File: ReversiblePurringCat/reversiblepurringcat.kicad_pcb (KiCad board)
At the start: 2 copper layers, 230.3 x 90.7 mm, 78 parts, among them J1 ScreenL, J2 ScreenR, SW0 SW_Push, SW1 SW_Push, SW10 SW_Push, SW11 SW_Push, SW12 SW_Push, SW13 SW_Push, SW14 SW_Push, SW15 SW_Push, SW16 SW_Push, SW17 SW_Push, SW18 SW_Push, SW19 SW_Push, SW2 SW_Push, SW20 SW_Push, SW21 SW_Push, SW22 SW_Push, SW23 SW_Push, SW24 SW_Push, SW25 SW_Push, SW26 SW_Push, SW27 SW_Push, SW28 SW_Push, SW29 SW_Push, SW3 SW_Push, SW30 SW_Push, SW31 SW_Push, SW4 SW_Push, SW5 SW_Push, SW6 SW_Push, SW7 SW_Push, SW8 SW_Push, SW9 SW_Push, U1 ProMicro-kbd, U2 ProMicro-kbd

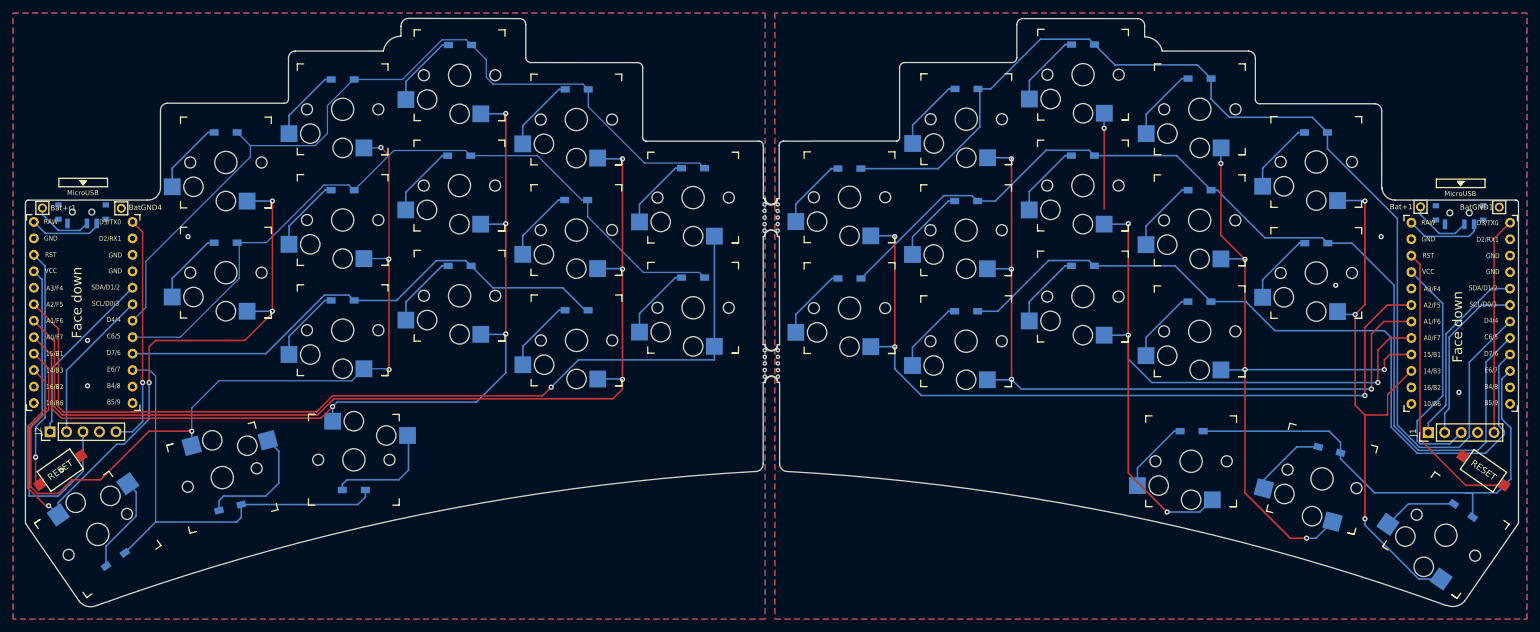
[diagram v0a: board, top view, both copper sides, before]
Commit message: reversible updates
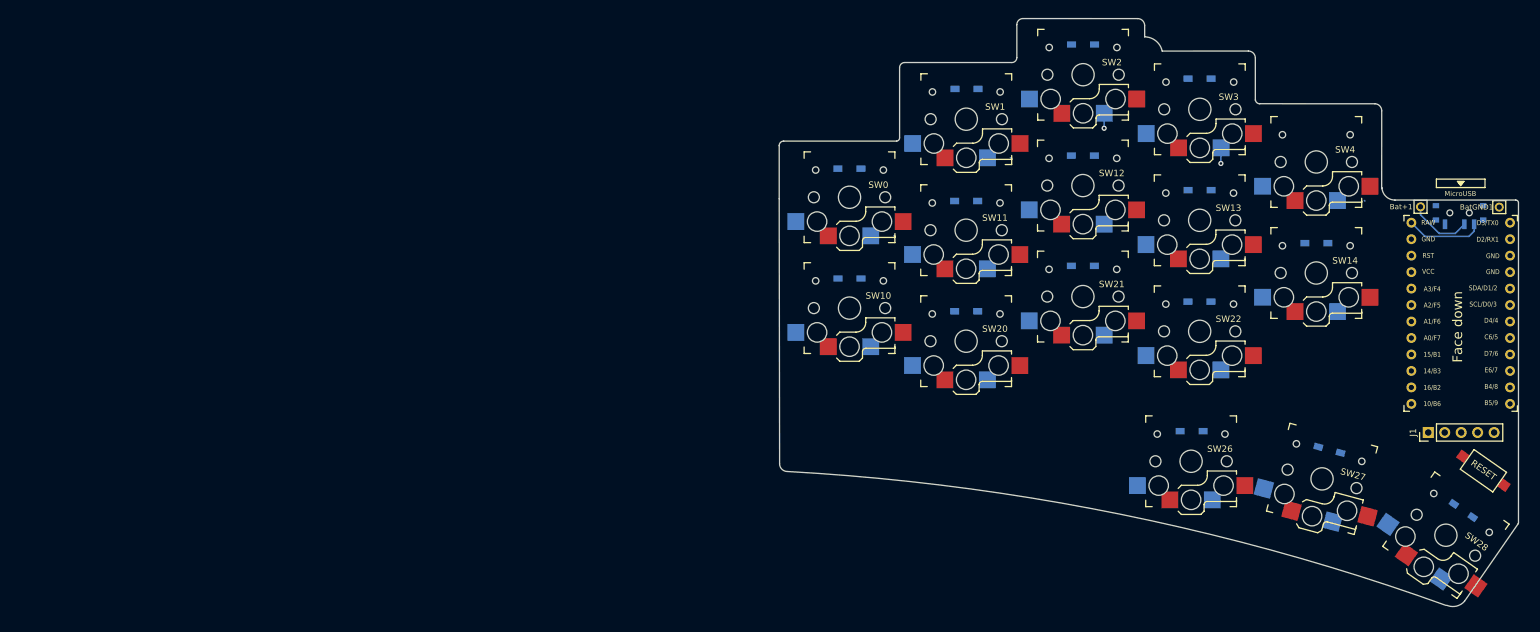
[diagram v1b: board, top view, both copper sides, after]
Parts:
- removed Bat+r1, BatGND4: MountingHole_Pad, kbd:1pin_conn
- removed D15, D16, D17, D18, D19, D23, D24, D25, D29, D30, D31, D4, D5, D6, D7, D8, D9: D, kbd:D3_SMD_v2
- removed J2: ScreenR, Connector_PinHeader_2.54mm:PinHeader_1x05_P2.54mm_Vertical
- removed RSW2: SW_Push, Button_Switch_SMD:SW_SPST_CK_RS282G05A3
- removed SW15, SW16, SW17, SW18, SW19, SW23, SW24, SW25, SW29, SW30, SW31, SW5, SW6, SW7, SW8, SW9: SW_Push, keyswitches:Kailh_socket_PG1350
- removed SW_POWER2: SW_SPDT, Button_Switch_SMD:SW_SPDT_PCM12
- removed U2: ProMicro-kbd, kbd:ProMicro_v3
- removed mouse-bite-2mm-slot (x2): VAL**, Duckyb-Parts:mouse-bite-5mm-slot-with-space-for-track
- SW0, SW1, SW10, SW11, SW12, SW13, SW14, SW2, SW20, SW21, SW22, SW26, SW27, SW28, SW3, SW4: footprint keyswitches:Kailh_socket_PG1350 -> keyswitches:Kailh_socket_PG1350_reversible
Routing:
- net row_0: track 175.1 -> 0.00 mm
- net row_1: track 155.3 -> 0.00 mm
- net col2r: track 151.5 -> 0.00 mm, vias 3 -> 0
- net col1r: track 141.6 -> 0.00 mm, vias 1 -> 0
- net col3r: track 139.6 -> 0.00 mm, vias 4 -> 0
- net col4r: track 133.1 -> 0.00 mm, vias 4 -> 0
- net col3: track 131.5 -> 2.43 mm, vias 5 -> 1
- net row_0r: track 128.1 -> 0.00 mm
- net col1: track 121.2 -> 0.23 mm, vias 3 -> 0
- net row_2: track 119.5 -> 0.00 mm
- net col2: track 116.9 -> 0.31 mm, vias 4 -> 0
- net row_1r: track 114.1 -> 0.00 mm
- net col5r: track 106.1 -> 0.00 mm, vias 4 -> 0
- net col4: track 107.5 -> 2.85 mm, vias 5 -> 1
- net col5: track 85.4 -> 0.73 mm, vias 3 -> 0
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- removed copper zone on B.Cu, net gnd
- removed copper zone on F.Cu, net gnd
- removed copper zone on B.Cu, net gnd_r
- removed copper zone on F.Cu, net gnd_r
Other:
- board size 230.3 x 90.7 mm -> 114 x 90.7 mm
- board text removed: "15/B1"
